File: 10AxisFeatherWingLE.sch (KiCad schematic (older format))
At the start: 19 parts, among them J1 feather long, J2 feather short, J3 feather long, J4 feather short, J5 grove connector, J6 feather breakout, U1 LSM9DS1, U2 BMP280

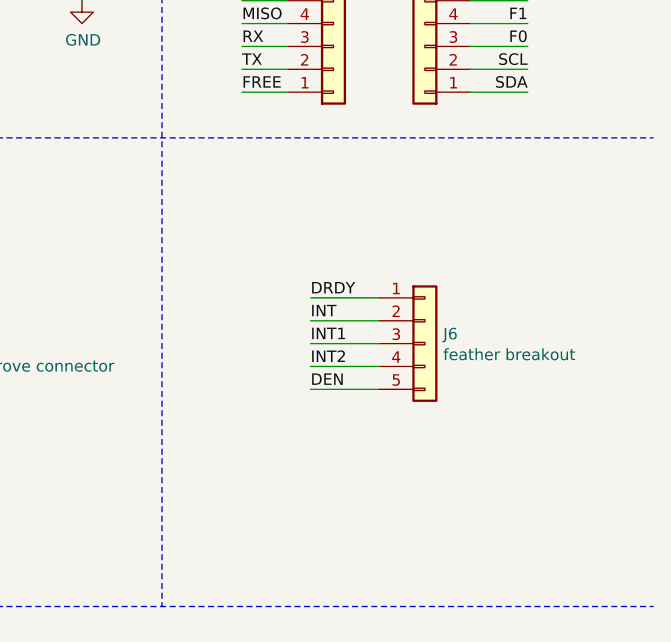
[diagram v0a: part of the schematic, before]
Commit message: Minor format fix
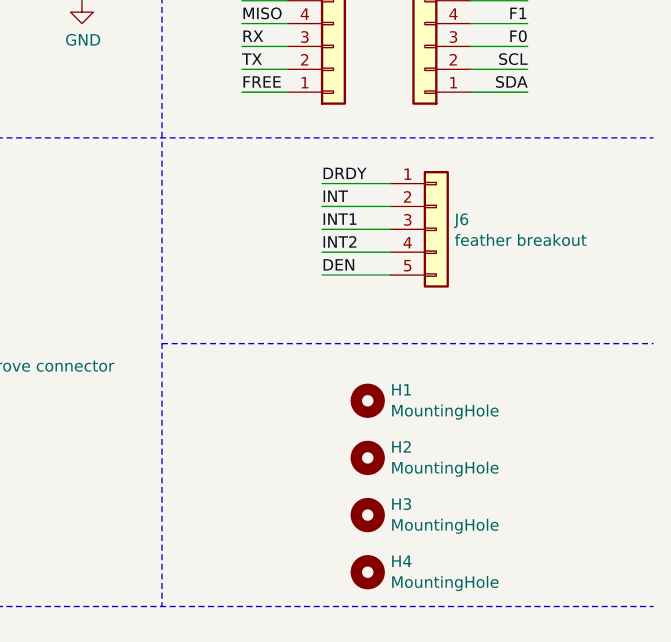
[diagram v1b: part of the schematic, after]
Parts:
- added H1, H2, H3, H4: MountingHole, MountingHole:MountingHole_2.7mm_M2.5, symbol Mechanical:MountingHole
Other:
- moved on the sheet: J6
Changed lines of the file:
@@
 L Connector_Generic:Conn_01x05 J6
 U 1 1 5E2059E9
-P 9500 5500
-F 0 "J6" H 9580 5542 50  0000 L CNN
-F 1 "feather breakout" H 9580 5451 50  0000 L CNN
-F 2 "Connector_PinHeader_2.54mm:PinHeader_1x05_P2.54mm_Vertical" H 9500 5500 50  0001 C CNN
-F 3 "~" H 9500 5500 50  0001 C CNN
-	1    9500 5500
-	1    0    0    -1
-$EndComp
-Text Label 9000 5300 0    50   ~ 0
+P 9550 5000
+F 0 "J6" H 9630 5042 50  0000 L CNN
+F 1 "feather breakout" H 9630 4951 50  0000 L CNN
+F 2 "Connector_PinHeader_2.54mm:PinHeader_1x05_P2.54mm_Vertical" H 9550 5000 50  0001 C CNN
+F 3 "~" H 9550 5000 50  0001 C CNN
+	1    9550 5000
+	1    0    0    -1
+$EndComp
+Text Label 9050 4800 0    50   ~ 0
 DRDY
-Text Label 9000 5400 0    50   ~ 0
+Text Label 9050 4900 0    50   ~ 0
 INT
-Text Label 9000 5500 0    50   ~ 0
+Text Label 9050 5000 0    50   ~ 0
 INT1
-Text Label 9000 5600 0    50   ~ 0
+Text Label 9050 5100 0    50   ~ 0
 INT2
-Text Label 9000 5700 0    50   ~ 0
+Text Label 9050 5200 0    50   ~ 0
 DEN
 Wire Wire Line
@@
 $EndComp
 Wire Wire Line
-	9000 5300 9300 5300
-Wire Wire Line
-	9000 5400 9300 5400
-Wire Wire Line
-	9000 5500 9300 5500
-Wire Wire Line
-	9000 5600 9300 5600
-Wire Wire Line
-	9000 5700 9300 5700
+	9050 4800 9350 4800
+Wire Wire Line
+	9050 4900 9350 4900
+Wire Wire Line
+	9050 5000 9350 5000
+Wire Wire Line
+	9050 5100 9350 5100
+Wire Wire Line
+	9050 5200 9350 5200
 Wire Wire Line
 	7000 5400 7300 5400
@@
 	1    0    0    -1
 $EndComp
+$Comp
+L Mechanical:MountingHole H1
+U 1 1 5E162FA6
+P 9250 5750
+F 0 "H1" H 9350 5796 50  0000 L CNN
+F 1 "MountingHole" H 9350 5705 50  0000 L CNN
+F 2 "MountingHole:MountingHole_2.7mm_M2.5" H 9250 5750 50  0001 C CNN
+F 3 "~" H 9250 5750 50  0001 C CNN
+	1    9250 5750
+	1    0    0    -1
+$EndComp
+$Comp
+L Mechanical:MountingHole H2
+U 1 1 5E163654
+P 9250 6000
+F 0 "H2" H 9350 6046 50  0000 L CNN
+F 1 "MountingHole" H 9350 5955 50  0000 L CNN
+F 2 "MountingHole:MountingHole_2.7mm_M2.5" H 9250 6000 50  0001 C CNN
+F 3 "~" H 9250 6000 50  0001 C CNN
+	1    9250 6000
+	1    0    0    -1
+$EndComp
+$Comp
+L Mechanical:MountingHole H3
+U 1 1 5E163A5D
+P 9250 6250
+F 0 "H3" H 9350 6296 50  0000 L CNN
+F 1 "MountingHole" H 9350 6205 50  0000 L CNN
+F 2 "MountingHole:MountingHole_2.7mm_M2.5" H 9250 6250 50  0001 C CNN
+F 3 "~" H 9250 6250 50  0001 C CNN
+	1    9250 6250
+	1    0    0    -1
+$EndComp
+$Comp
+L Mechanical:MountingHole H4
+U 1 1 5E163E72
+P 9250 6500
+F 0 "H4" H 9350 6546 50  0000 L CNN
+F 1 "MountingHole" H 9350 6455 50  0000 L CNN
+F 2 "MountingHole:MountingHole_2.7mm_M2.5" H 9250 6500 50  0001 C CNN
+F 3 "~" H 9250 6500 50  0001 C CNN
+	1    9250 6500
+	1    0    0    -1
+$EndComp
+Wire Notes Line
+	8350 5500 10500 5500
 $EndSCHEMATC
